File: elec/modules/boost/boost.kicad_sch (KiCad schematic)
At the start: 9 parts, among them J1 Conn_01x05, J2 Conn_01x05, U1 LM2587S-ADJ

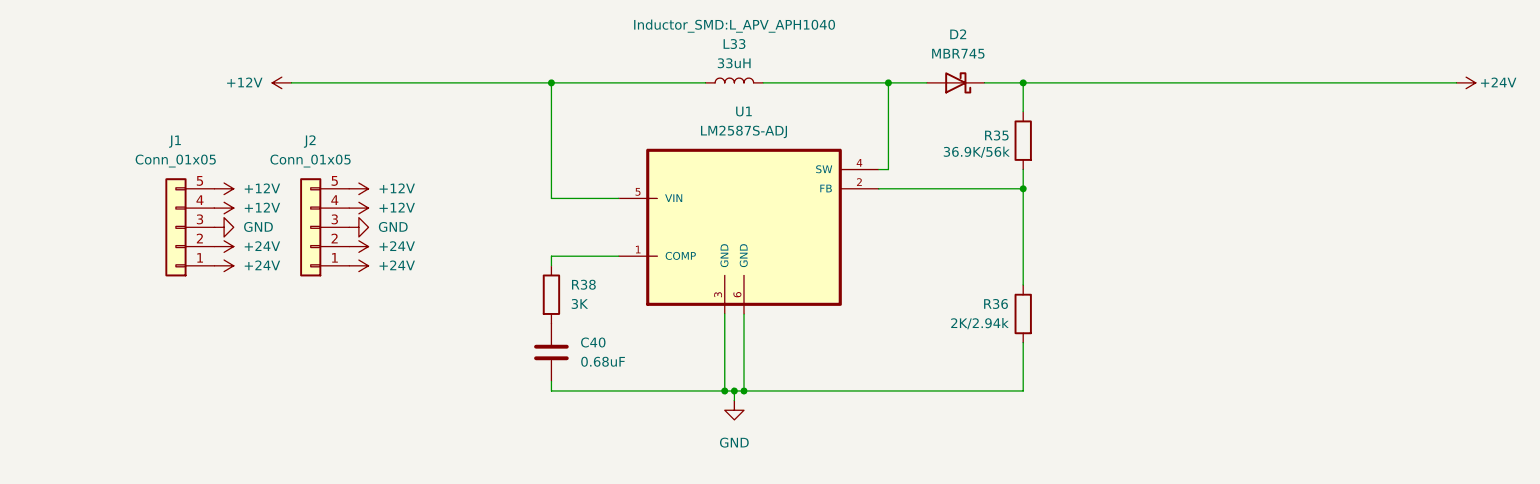
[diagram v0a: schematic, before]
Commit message: sleepy but did most pcbs
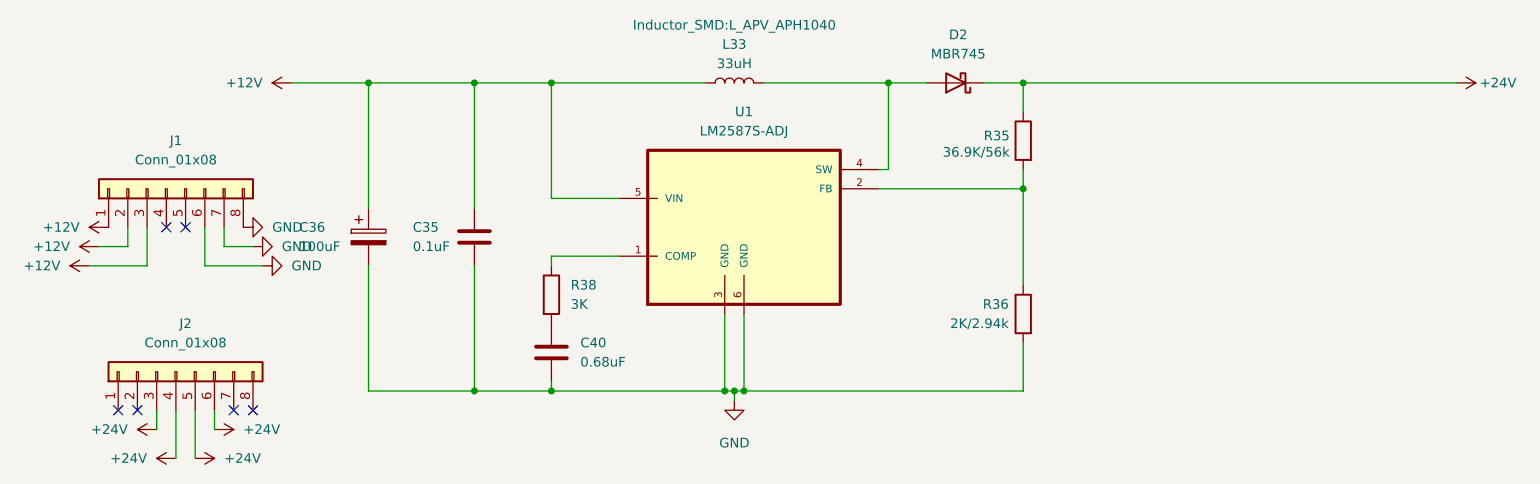
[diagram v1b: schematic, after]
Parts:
- removed J1, J2: Conn_01x05, Pinheaders:PinHeader_1x05_P2.54mm_Vertical, symbol Connector_Generic:Conn_01x05
- added C35: 0.1uF, Capacitor_SMD:C_0603_1608Metric, symbol Device:C
- added C36: 100uF, Capacitor_THT:CP_Radial_D8.0mm_P3.50mm, symbol Device:C_Polarized
- added J1, J2: Conn_01x08, Pinheaders:PinHeader_1x08_P2.54mm_Vertical, symbol Connector_Generic:Conn_01x08
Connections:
- net +12V: now also C35.1, C36.1, J1.1 (Pin_1), J1.2 (Pin_2), J1.3 (Pin_3)
- net +24V: now also J2.3 (Pin_3), J2.4 (Pin_4), J2.5 (Pin_5), J2.6 (Pin_6)
- net GND: now also C35.2, C36.2, J1.6 (Pin_6), J1.7 (Pin_7), J1.8 (Pin_8)
- no-connect marks 0 -> 6
